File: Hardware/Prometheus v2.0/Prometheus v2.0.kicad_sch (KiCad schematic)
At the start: 44 parts, among them IC1 LSF0108PWR, J1 PJ-002A, J2 Conn_01x02_Socket, J3 Conn_01x08_Pin, K1 SRD-05VDC-SL-C, Q1 IRLML6246, Q2 IRLML6246, Q3 IRLML6246, U1 LMS1585ACT-3.3_NOPB, U2 LM7805_TO220, U3 MQ-135, U4 DHT-11

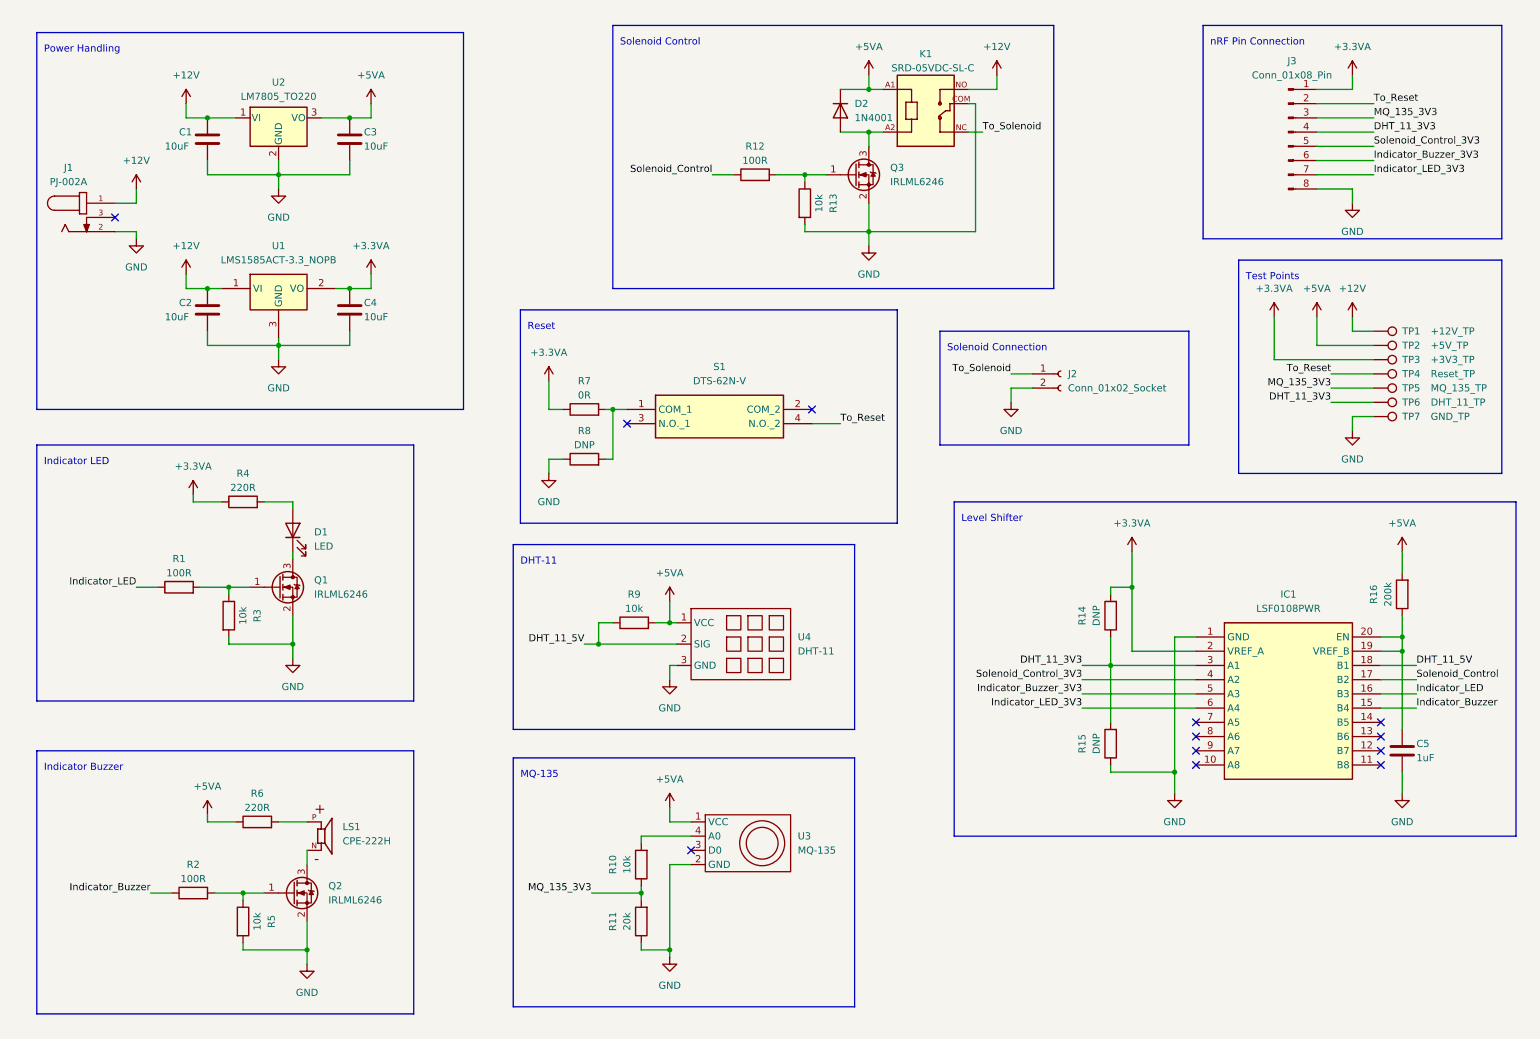
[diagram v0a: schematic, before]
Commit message: v2.1
- First design completion
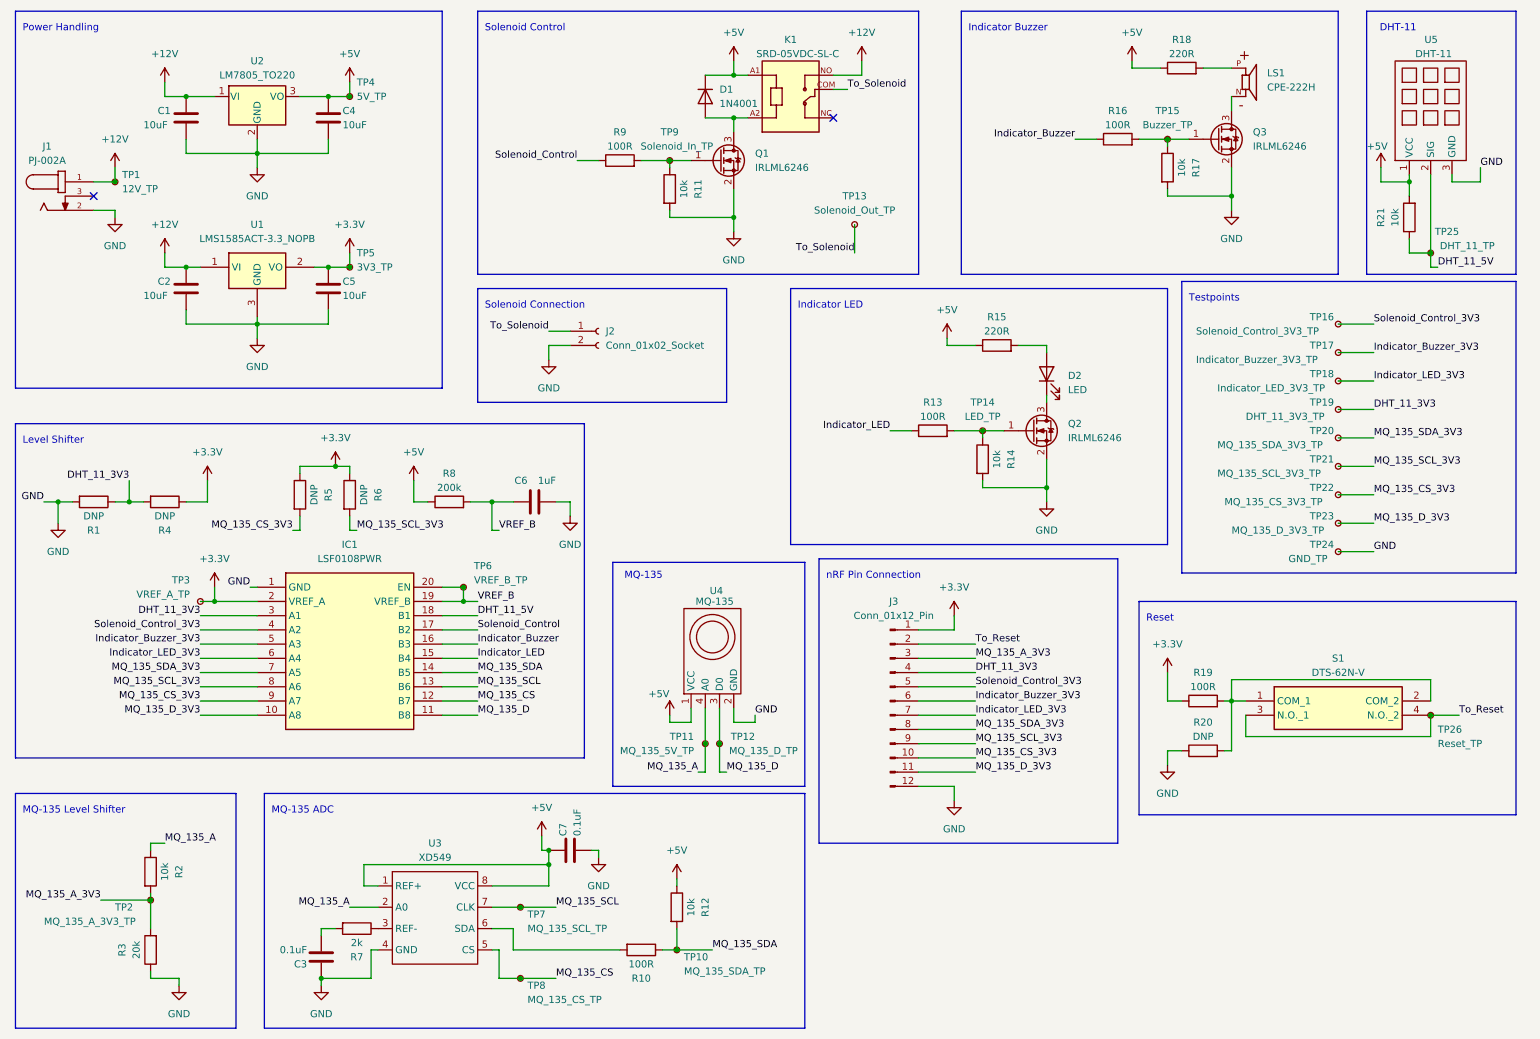
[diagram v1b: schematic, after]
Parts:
- removed C5: 1uF, symbol Device:C
- removed J3: Conn_01x08_Pin, symbol Connector:Conn_01x08_Pin
- removed R11: 20k, symbol Device:R
- removed R16: 200k, symbol Device:R
- removed R9: 10k, symbol Device:R
- removed TP1: +12V_TP, symbol Connector:TestPoint
- removed TP2: +5V_TP, symbol Connector:TestPoint
- removed TP3: +3V3_TP, symbol Connector:TestPoint
- removed TP4: Reset_TP, symbol Connector:TestPoint
- removed TP5: MQ_135_TP, symbol Connector:TestPoint
- removed TP6: DHT_11_TP, symbol Connector:TestPoint
- removed TP7: GND_TP, symbol Connector:TestPoint
- removed U3: MQ-135, symbol Sensors:MQ-135
- removed U4: DHT-11, symbol Sensors:DHT-11
- added C3, C7: 0.1uF, Capacitor_SMD:C_0805_2012Metric, symbol Device:C
- added C6: 1uF, Capacitor_SMD:C_0805_2012Metric, symbol Device:C
- added J3: Conn_01x12_Pin, Connector_PinHeader_2.54mm:PinHeader_1x12_P2.54mm_Horizontal, symbol Connector:Conn_01x12_Pin
- added R12, R2, R21: 10k, Resistor_SMD:R_0805_2012Metric, symbol Device:R
- added R3: 20k, Resistor_SMD:R_0805_2012Metric, symbol Device:R
- added R5, R6: DNP, Resistor_SMD:R_0805_2012Metric, symbol Device:R
- added R7: 2k, Resistor_SMD:R_0805_2012Metric, symbol Device:R
- added R8: 200k, Resistor_SMD:R_0805_2012Metric, symbol Device:R
- added TP1: 12V_TP, TestPoint:TestPoint_Pad_1.0x1.0mm, symbol Connector:TestPoint_Small
- added TP10: MQ_135_SDA_TP, TestPoint:TestPoint_Pad_1.0x1.0mm, symbol Connector:TestPoint_Small
- added TP11: MQ_135_5V_TP, TestPoint:TestPoint_Pad_1.0x1.0mm, symbol Connector:TestPoint_Small
- added TP12: MQ_135_D_TP, TestPoint:TestPoint_Pad_1.0x1.0mm, symbol Connector:TestPoint_Small
- added TP13: Solenoid_Out_TP, TestPoint:TestPoint_Pad_1.0x1.0mm, symbol Connector:TestPoint_Small
- added TP14: LED_TP, TestPoint:TestPoint_Pad_1.0x1.0mm, symbol Connector:TestPoint_Small
- added TP15: Buzzer_TP, TestPoint:TestPoint_Pad_1.0x1.0mm, symbol Connector:TestPoint_Small
- added TP16: Solenoid_Control_3V3_TP, TestPoint:TestPoint_Pad_1.0x1.0mm, symbol Connector:TestPoint_Small
- added TP17: Indicator_Buzzer_3V3_TP, TestPoint:TestPoint_Pad_1.0x1.0mm, symbol Connector:TestPoint_Small
- added TP18: Indicator_LED_3V3_TP, TestPoint:TestPoint_Pad_1.0x1.0mm, symbol Connector:TestPoint_Small
- added TP19: DHT_11_3V3_TP, TestPoint:TestPoint_Pad_1.0x1.0mm, symbol Connector:TestPoint_Small
- added TP2: MQ_135_A_3V3_TP, TestPoint:TestPoint_Pad_1.0x1.0mm, symbol Connector:TestPoint_Small
- added TP20: MQ_135_SDA_3V3_TP, TestPoint:TestPoint_Pad_1.0x1.0mm, symbol Connector:TestPoint_Small
- added TP21: MQ_135_SCL_3V3_TP, TestPoint:TestPoint_Pad_1.0x1.0mm, symbol Connector:TestPoint_Small
- added TP22: MQ_135_CS_3V3_TP, TestPoint:TestPoint_Pad_1.0x1.0mm, symbol Connector:TestPoint_Small
- added TP23: MQ_135_D_3V3_TP, TestPoint:TestPoint_Pad_1.0x1.0mm, symbol Connector:TestPoint_Small
- added TP24: GND_TP, TestPoint:TestPoint_Pad_2.0x2.0mm, symbol Connector:TestPoint_Small
- added TP25: DHT_11_TP, TestPoint:TestPoint_Pad_1.0x1.0mm, symbol Connector:TestPoint_Small
- added TP26: Reset_TP, TestPoint:TestPoint_Pad_1.0x1.0mm, symbol Connector:TestPoint_Small
- added TP3: VREF_A_TP, TestPoint:TestPoint_Pad_1.0x1.0mm, symbol Connector:TestPoint_Small
- added TP4: 5V_TP, TestPoint:TestPoint_Pad_1.0x1.0mm, symbol Connector:TestPoint_Small
- added TP5: 3V3_TP, TestPoint:TestPoint_Pad_1.0x1.0mm, symbol Connector:TestPoint_Small
- added TP6: VREF_B_TP, TestPoint:TestPoint_Pad_1.0x1.0mm, symbol Connector:TestPoint_Small
- added TP7: MQ_135_SCL_TP, TestPoint:TestPoint_Pad_1.0x1.0mm, symbol Connector:TestPoint_Small
- added TP8: MQ_135_CS_TP, TestPoint:TestPoint_Pad_1.0x1.0mm, symbol Connector:TestPoint_Small
- added TP9: Solenoid_In_TP, TestPoint:TestPoint_Pad_1.0x1.0mm, symbol Connector:TestPoint_Small
- added U3: XD549, Package_DIP:DIP-8_W7.62mm, symbol ADC:XD549
- added U4: MQ-135, symbol Sensors:MQ-135
- added U5: DHT-11, symbol Sensors:DHT-11
- C1, C2: footprint (none) -> Capacitor_SMD:C_0805_2012Metric; JLCPCB (none) -> https://jlcpcb.com/partdetail/Yageo-CC0805KKX5R6BB106/C89832
- C4: renamed from C3; footprint (none) -> Capacitor_SMD:C_0805_2012Metric; JLCPCB (none) -> https://jlcpcb.com/partdetail/Yageo-CC0805KKX5R6BB106/C89832
- C5: renamed from C4; footprint (none) -> Capacitor_SMD:C_0805_2012Metric; JLCPCB (none) -> https://jlcpcb.com/partdetail/Yageo-CC0805KKX5R6BB106/C89832
- D1: renamed from D2; JLCPCB (none) -> https://jlcpcb.com/partdetail/VishayIntertech-1N4001_E373/C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
- D2: renamed from D1; footprint (none) -> LED_THT:LED_D3.0mm_FlatTop; JLCPCB (none) -> https://jlcpcb.com/partdetail/EverlightElec-333_2SURD_S530_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
- IC1: JLCPCB (none) -> https://jlcpcb.com/partdetail/Nexperia-LSF0108PWQ100J/C5515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
- J1: JLCPCB (none) -> https://jlcpcb.com/partdetail/Jinjia-DC02IB/C718035
- K1: JLCPCB (none) -> https://jlcpcb.com/partdetail/Ningbo_SongleRelay-SRA_05VDCC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
- LS1: footprint CPE-222H:CUI_CPE-222H -> Buzzer_Beeper:MagneticBuzzer_StarMicronics_HMB-06_HMB-12; JLCPCB (none) -> https://jlcpcb.com/partdetail/Jiangsu_HuanengElec-HMB120605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
- Q1: renamed from Q3; JLCPCB (none) -> https://jlcpcb.com/partdetail/InfineonTechnologies-IRLML624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
- Q2: renamed from Q1; JLCPCB (none) -> https://jlcpcb.com/partdetail/InfineonTechnologies-IRLML624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
- Q3: renamed from Q2; JLCPCB (none) -> https://jlcpcb.com/partdetail/InfineonTechnologies-IRLML624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
- R1: renamed from R15; footprint (none) -> Resistor_SMD:R_0805_2012Metric
- R10: value 10k -> 100R; footprint (none) -> Resistor_SMD:R_0805_2012Metric; JLCPCB (none) -> https://jlcpcb.com/partdetail/Yageo-AC0805JR7W100RL/C728002
- R11: renamed from R13; footprint (none) -> Resistor_SMD:R_0805_2012Metric; JLCPCB (none) -> https://jlcpcb.com/partdetail/Yageo-AC0805JR0710KL/C138260
- R13: renamed from R1; footprint (none) -> Resistor_SMD:R_0805_2012Metric; JLCPCB (none) -> https://jlcpcb.com/partdetail/Yageo-AC0805JR7W100RL/C728002
- R14: renamed from R3; footprint (none) -> Resistor_SMD:R_0805_2012Metric; JLCPCB (none) -> https://jlcpcb.com/partdetail/Yageo-AC0805JR0710KL/C138260
- R15: renamed from R4; footprint (none) -> Resistor_SMD:R_0805_2012Metric; JLCPCB (none) -> https://jlcpcb.com/partdetail/Kamaya-RPCH20K221JTP/C340559
- R16: renamed from R2; footprint (none) -> Resistor_SMD:R_0805_2012Metric; JLCPCB (none) -> https://jlcpcb.com/partdetail/Yageo-AC0805JR7W100RL/C728002
- R17: renamed from R5; footprint (none) -> Resistor_SMD:R_0805_2012Metric; JLCPCB (none) -> https://jlcpcb.com/partdetail/Yageo-AC0805JR0710KL/C138260
- R18: renamed from R6; footprint (none) -> Resistor_SMD:R_0805_2012Metric; JLCPCB (none) -> https://jlcpcb.com/partdetail/Kamaya-RPCH20K221JTP/C340559
- R19: renamed from R7; value 0R -> 100R; footprint (none) -> Resistor_SMD:R_0805_2012Metric; JLCPCB (none) -> https://jlcpcb.com/partdetail/Yageo-AC0805JR7W100RL/C728002
- R20: renamed from R8; footprint (none) -> Resistor_SMD:R_0805_2012Metric
- R4: renamed from R14; footprint (none) -> Resistor_SMD:R_0805_2012Metric
- R9: renamed from R12; footprint (none) -> Resistor_SMD:R_0805_2012Metric; JLCPCB (none) -> https://jlcpcb.com/partdetail/Yageo-AC0805JR7W100RL/C728002
- S1: JLCPCB (none) -> https://jlcpcb.com/partdetail/Diptronics-DTSA_65NV/C224975
- U1: JLCPCB (none) -> https://jlcpcb.com/partdetail/TexasInstruments-LMS1585ACT_3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
- U2: JLCPCB (none) -> https://jlcpcb.com/partdetail/6334298-LM7805CT/C5444281
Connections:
- net MQ_135_3V3 is gone; now on net MQ_135_SDA: R10.1
- net +12V: now also TP1.1
- net DHT_11_3V3: now also R1.1, R4.2, J3.4 (Pin_4), TP19.1; no longer R1.2, R4.1
- net DHT_11_5V: now also R21.1, TP25.1, U5.2 (SIG)
- net GND: now also R1.2, C3.1, C6.2, C7.2, J3.12 (Pin_12), R3.1, TP24.1, U3.4 (GND), U4.2 (GND), U5.3 (GND); no longer K1.COM, R1.1
- net Indicator_Buzzer: now also IC1.16 (B3); no longer IC1.15 (B4)
- net Indicator_Buzzer_3V3: now also J3.6 (Pin_6), TP17.1
- net Indicator_LED: now also IC1.15 (B4); no longer IC1.16 (B3)
- net Indicator_LED_3V3: now also J3.7 (Pin_7), TP18.1
- net Solenoid_Control_3V3: now also J3.5 (Pin_5), TP16.1
- net To_Reset: now also S1.3 (N.O._1), J3.2 (Pin_2), TP26.1
- net To_Solenoid: now also K1.COM, TP13.1; no longer K1.NC
- net at R19.2, R20.2, S1.1 (COM_1): now also S1.2 (COM_2)
- net at Q2.1 (G), R13.2, R14.1: now also TP14.1
- net at Q3.1 (G), R16.2, R17.1: now also TP15.1
- net at Q1.1 (G), R11.1, R9.2: now also TP9.1
- net VREF_B: now reaches IC1.19 (VREF_B), IC1.20 (EN)
- net VREF_B: now also C6.1, R8.2, TP6.1
- net MQ_135_D_3V3: now reaches IC1.10 (A8)
- net MQ_135_D_3V3: now also J3.11 (Pin_11), TP23.1
- net MQ_135_D: now reaches IC1.11 (B8)
- net MQ_135_D: now also TP12.1, U4.3 (D0)
- net MQ_135_CS: now reaches IC1.12 (B7)
- net MQ_135_CS: now also TP8.1, U3.5 (CS)
- net MQ_135_SCL: now reaches IC1.13 (B6)
- net MQ_135_SCL: now also TP7.1, U3.7 (CLK)
- net MQ_135_SDA: now reaches IC1.14 (B5)
- net MQ_135_SDA: now also R12.2, TP10.1
- net MQ_135_SDA_3V3: now reaches IC1.7 (A5)
- net MQ_135_SDA_3V3: now also J3.8 (Pin_8), TP20.1
- net MQ_135_SCL_3V3: now reaches IC1.8 (A6)
- net MQ_135_SCL_3V3: now also J3.9 (Pin_9), R6.2, TP21.1
- net MQ_135_CS_3V3: now reaches IC1.9 (A7)
- net MQ_135_CS_3V3: now also J3.10 (Pin_10), R5.2, TP22.1
- net at R10.2: now also U3.6 (SDA)
- net +3.3VA renamed +3.3V
- net +3.3V: now also R4.1, J3.1 (Pin_1), R5.1, R6.1, TP3.1, TP5.1; no longer R15.1, R4.2
- net +5VA renamed +5V
- net +5V: now also R15.1, C7.1, R12.1, R21.2, R8.1, TP4.1, U3.1 (REF+), U3.8 (VCC), U4.1 (VCC), U5.1 (VCC)
- new net: R7.1, U3.3 (REF-)
- new net: C3.2, R7.2
- new net MQ_135_A: R2.1, TP11.1, U3.2 (A0), U4.4 (A0)
- new net MQ_135_A_3V3: J3.3 (Pin_3), R2.2, R3.2, TP2.1
- no-connect marks 12 -> 2
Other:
- note added: "MQ-135 ADC"
- note added: "MQ-135 Level Shifter"
- note added: "Testpoints"
- note removed: "Test Points"
- moved on the sheet: C1, C2, C4, C5, D1, D2, IC1, J1, J2, K1, LS1, Q1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
